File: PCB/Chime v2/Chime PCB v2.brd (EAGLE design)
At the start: 62.2 x 77.6 mm, 34 parts, among them J1_I2C1 1725672, J2_I2C 1725672, J4_A1 282834-3, J5_A0 282834-3, U1 MS5803-02BA, X4 BQ24074

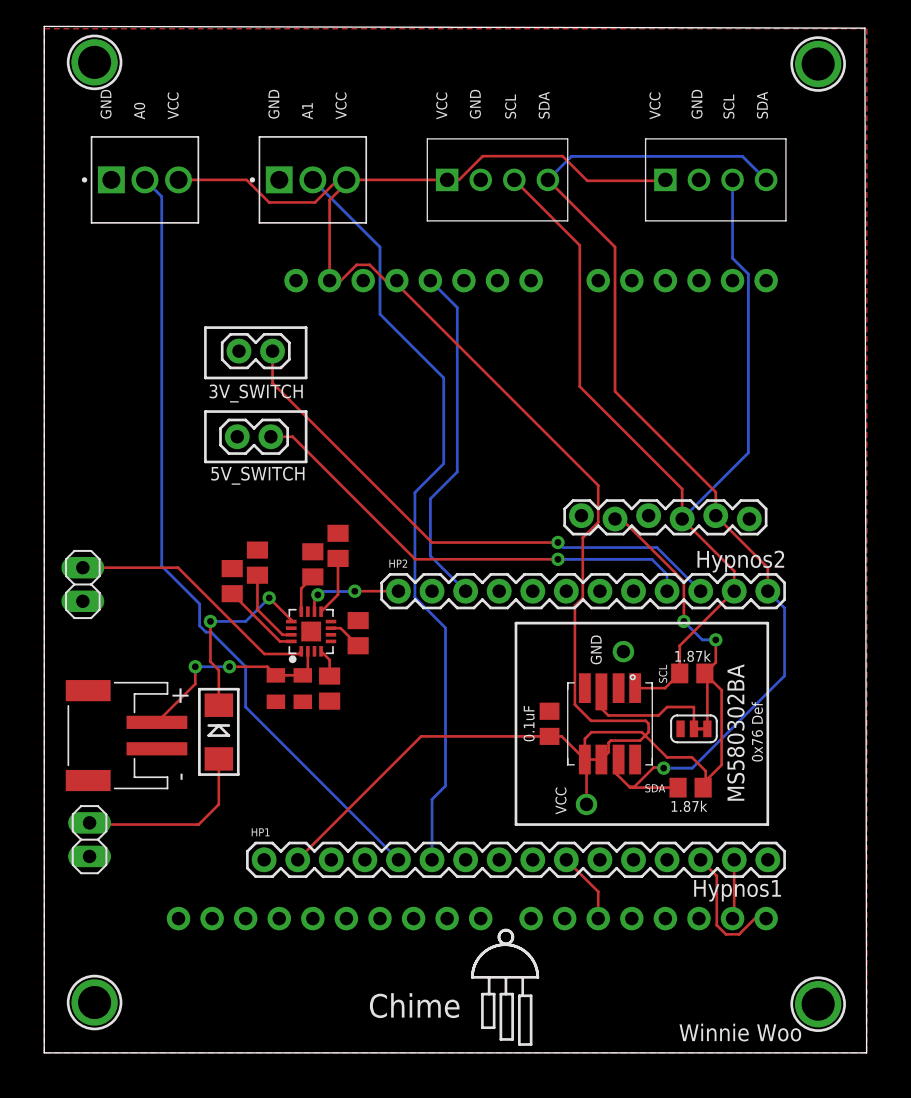
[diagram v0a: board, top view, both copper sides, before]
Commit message: Add files via upload
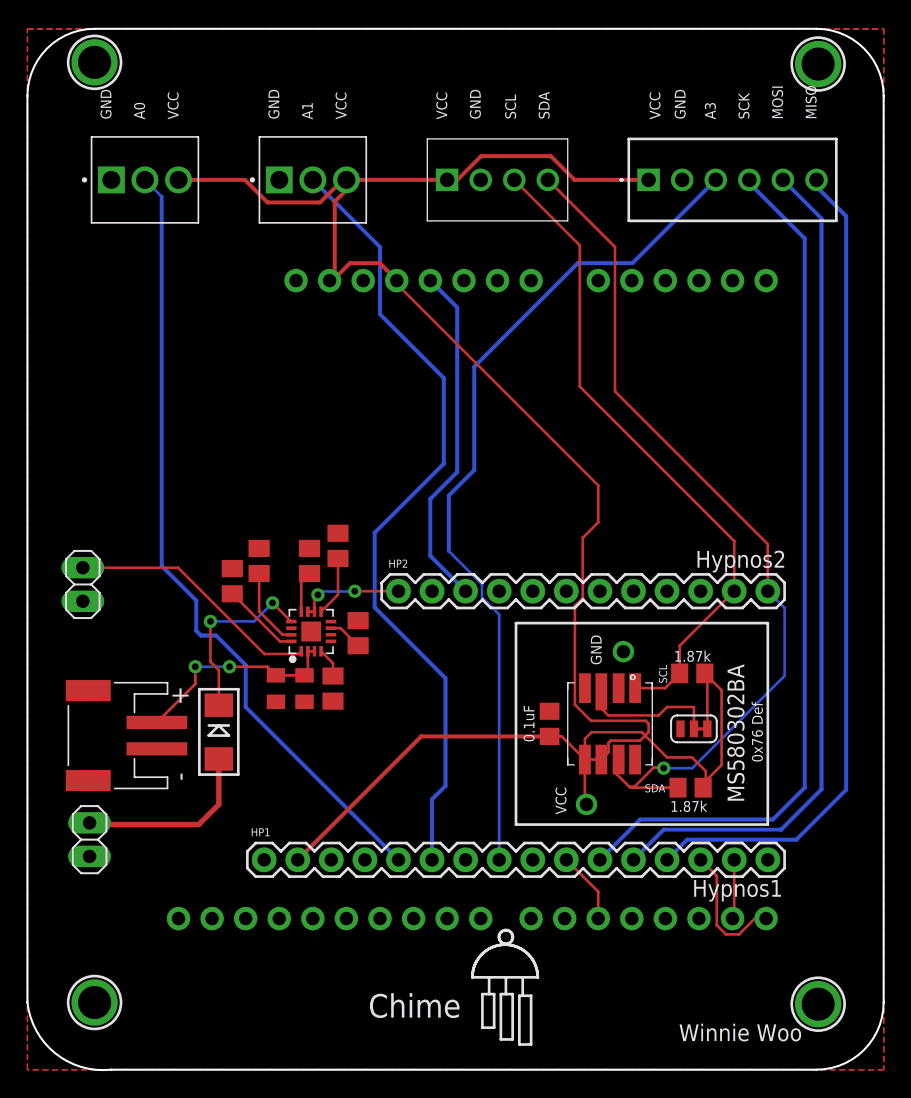
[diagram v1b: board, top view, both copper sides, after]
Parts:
- removed J1_I2C1: 1725672, 1725672:1725672
- removed J6_TSL2591: (no value), SparkFun-Connectors:1X06_LOCK
- removed J7_S3V, J8_S5V: (no value), SparkFun-Connectors:1X02
- added J1_SPI: 1725698, 1725698:1725698
- moved R3 0.36 mm to (20.1, 37.2)
- moved R8 0.25 mm to (21.8, 27.6)
- moved R4 0.18 mm to (16.3, 37.2)
- moved C5 0.13 mm to (19.7, 27.6)
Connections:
- removed net INT: J6_TSL2591.6
- removed net VIN: J6_TSL2591.1
- net 3VSWITCH: no longer J7_S3V.1
- net 5VSWITCH: no longer J8_S5V.1
- net A3: now also J1_SPI.3
- net GND: now also J1_SPI.2; no longer J1_I2C1.2, J6_TSL2591.3, J7_S3V.2, J8_S5V.2
- net MISO: now also J1_SPI.6
- net MOSI: now also J1_SPI.5
- net SCK: now also J1_SPI.4
- net SCL: no longer J1_I2C1.3, J6_TSL2591.4
- net SDA: no longer J1_I2C1.4, J6_TSL2591.5
- net VCC: now also J1_SPI.1; no longer J1_I2C1.1, J6_TSL2591.2
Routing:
- net SCK: track 0.00 -> 65.5 mm
- net A3: track 0.00 -> 63.8 mm
- net MOSI: track 0.00 -> 63.7 mm
- net MISO: track 0.00 -> 62.8 mm
- net 3VSWITCH: track 41.3 -> 0.00 mm, vias 1 -> 0
- net 5VSWITCH: track 35.6 -> 0.00 mm, vias 1 -> 0
- net SCL: track 78.0 -> 49.8 mm
- net SDA: track 84.4 -> 66.4 mm
- net VCC: track 179.0 -> 161.6 mm, vias 2 -> 0
- net A1: track 57.8 -> 60.3 mm
- net VLIPO: track 15.8 -> 16.4 mm
- added copper zone on layer 16, net VCC
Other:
- board size 62.2 x 77.6 mm -> 64.8 x 78.8 mm
- board text added: "A3"
- board text added: "MISO"
- board text added: "MOSI"
- board text added: "SCK"
- board text removed: "3V_SWITCH"
- board text removed: "5V_SWITCH"
